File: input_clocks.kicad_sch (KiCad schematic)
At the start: 86 parts, among them J201 REFIN, J202 REFIN_DIRECT_P, J203 REFIN_DIRECT_N, J208 VTUNE, T201 TC2-1T+, U203 TSV914, U204 74LVC1G66, X201 XTCLH40M000CHJA0P0

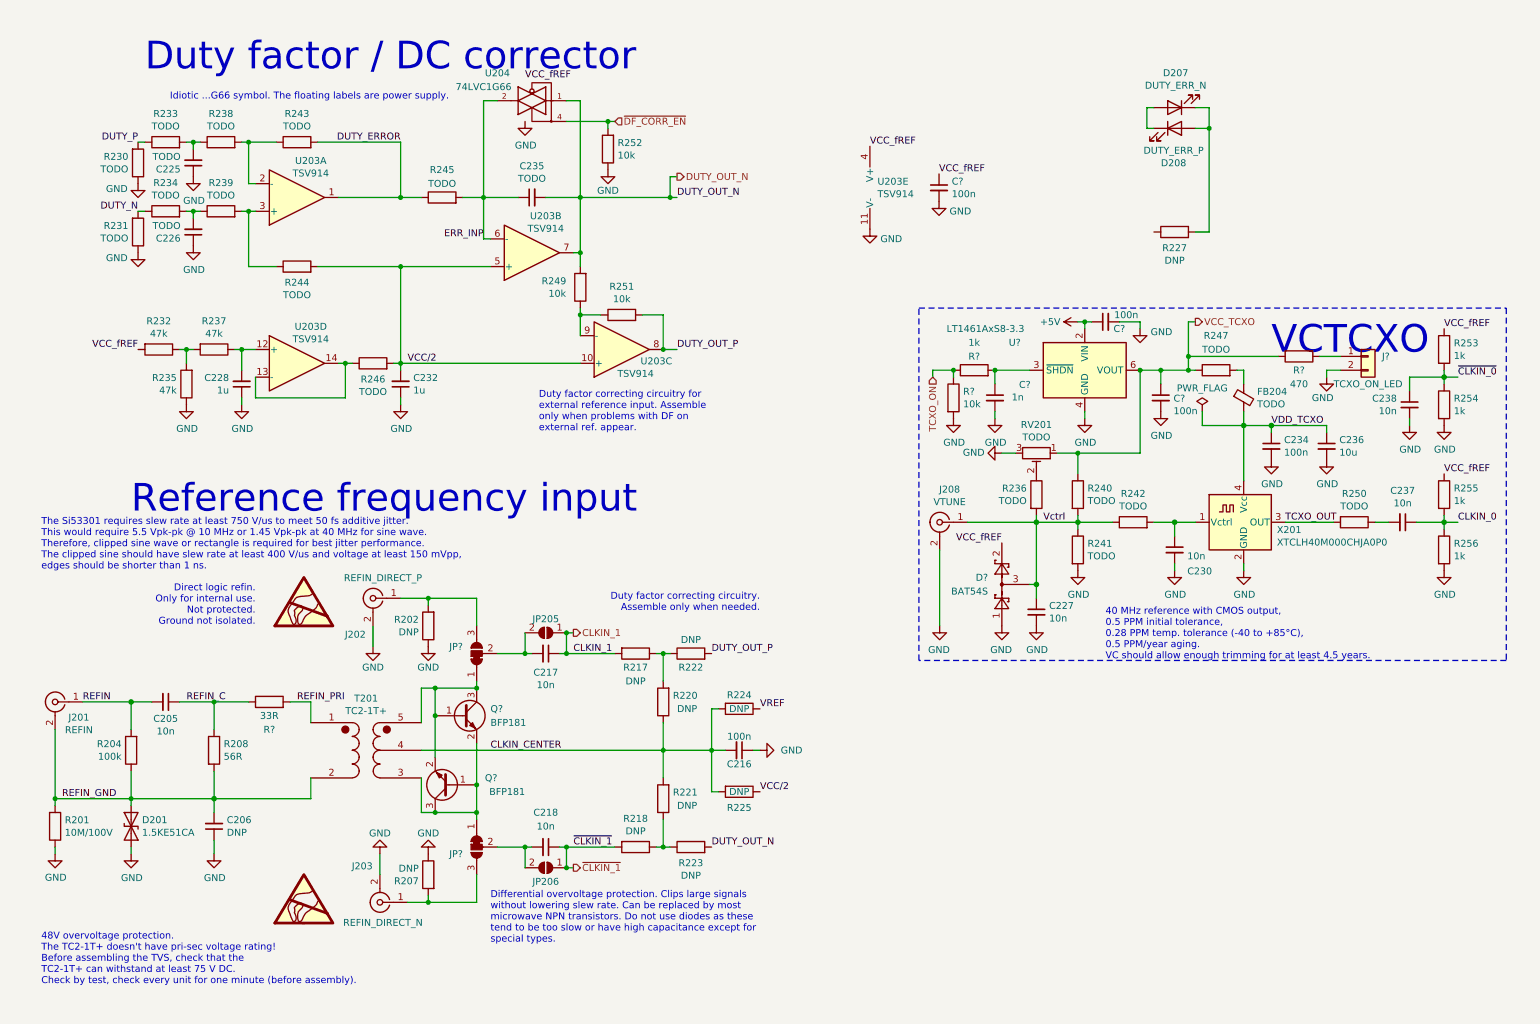
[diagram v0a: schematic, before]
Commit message: Updated schematics
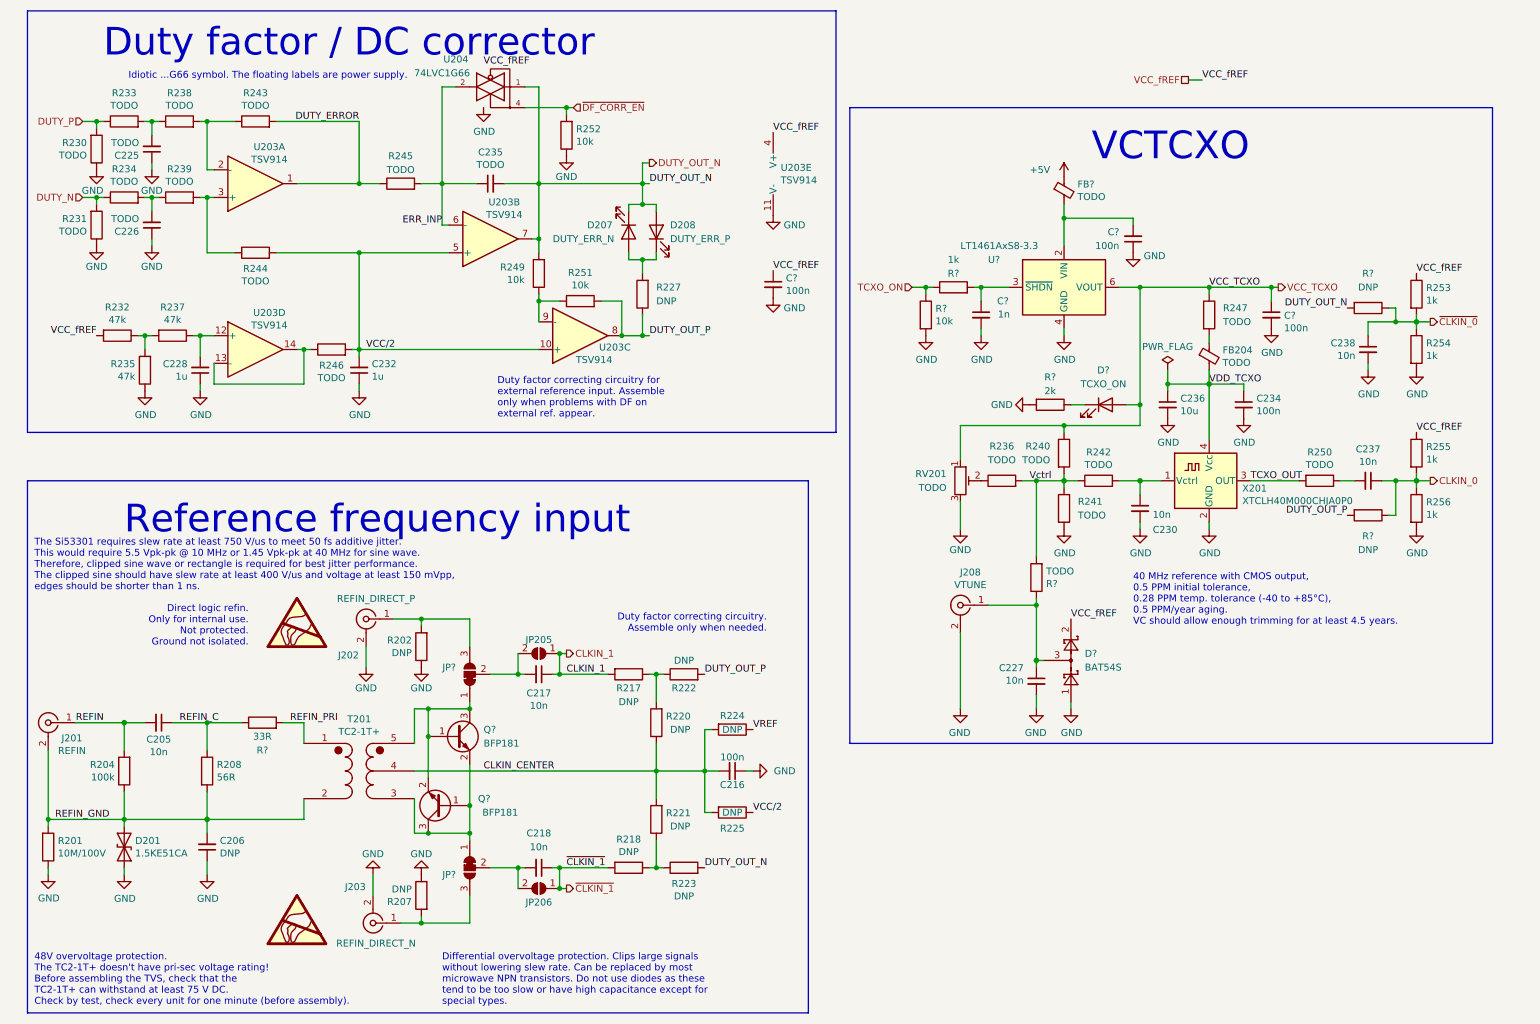
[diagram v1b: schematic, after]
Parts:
- removed J?: TCXO_ON_LED, symbol Connector_Generic:Conn_01x02
- added D?: TCXO_ON, LED_SMD:LED_0603_1608Metric_Pad1.05x0.95mm_HandSolder, symbol Device:LED
- added FB?: TODO, Inductor_SMD:L_0603_1608Metric_Pad1.05x0.95mm_HandSolder, symbol Device:FerriteBead_Small
- added R? (x2): DNP, Resistor_SMD:R_0603_1608Metric_Pad0.98x0.95mm_HandSolder, symbol Device:R
- added R?: TODO, Resistor_SMD:R_0603_1608Metric_Pad0.98x0.95mm_HandSolder, symbol Device:R
- R?: value 470 -> 2k
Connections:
- net +5V: now also FB?.1; no longer C?.1, U?.2 (VIN)
- net CLKIN_0: now also R?.1
- net DUTY_OUT_N: now also D207.1 (K), D208.2 (A), R?.2
- net DUTY_OUT_P: now also R227.1, R?.2
- net GND: now also C?.1, R?.2; no longer C?.2
- net VCC_TCXO: now also D?.2 (A); no longer R?.2
- net Vctrl: now also R?.2; no longer C227.1, D?.3, J208.1 (In)
- net ~{CLKIN_0}: now also R?.1
- net at R?.1: now also D?.1 (K)
- net at D207.2 (A), D208.1 (K): now also R227.2
- new net: C227.1, D?.3, J208.1 (In), R?.1
- new net: C?.2, FB?.2, U?.2 (VIN)
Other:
- moved on the sheet: C205, C206, C216, C217, C218, C225, C226, C227, C228, C230, C232, C234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
